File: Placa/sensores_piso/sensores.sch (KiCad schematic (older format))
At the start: 10 parts, among them P1 CONN_8X2, U1 CNY70, U2 CNY70

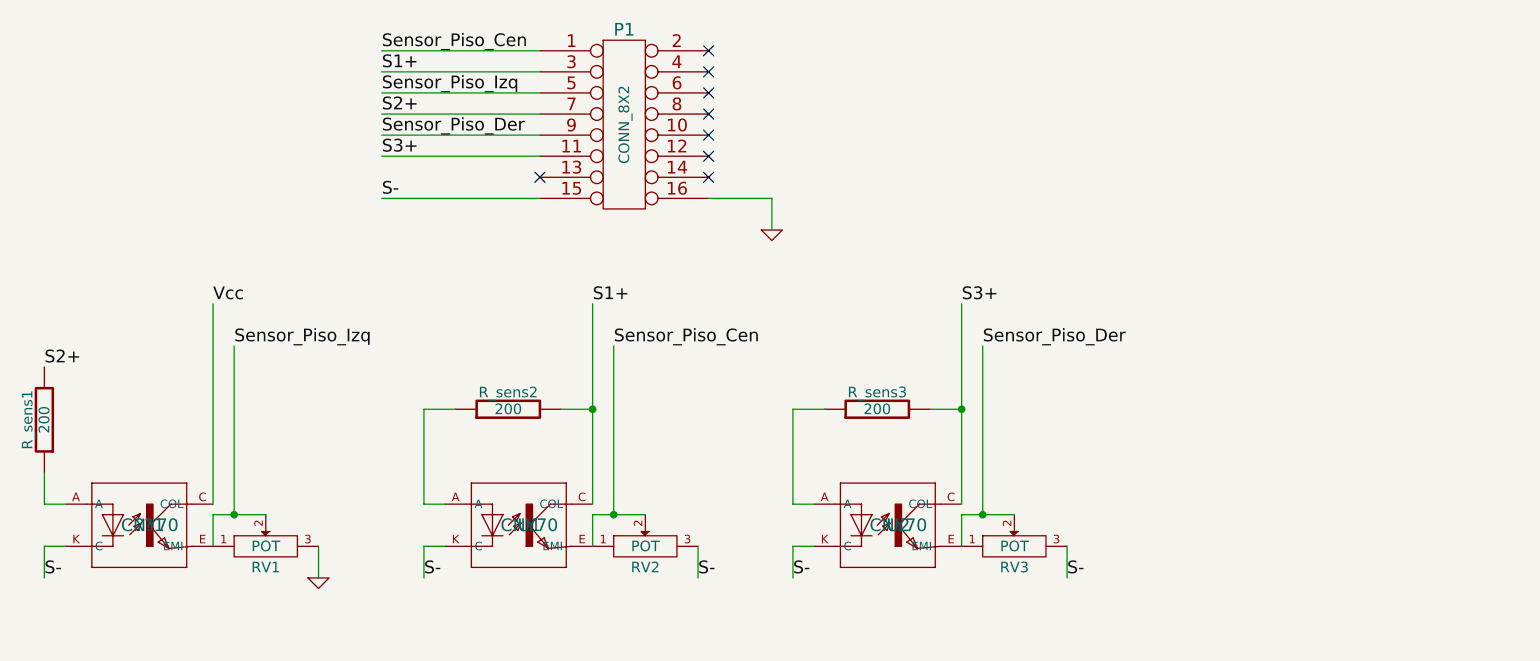
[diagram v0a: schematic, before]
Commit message: arreglo placa sensores
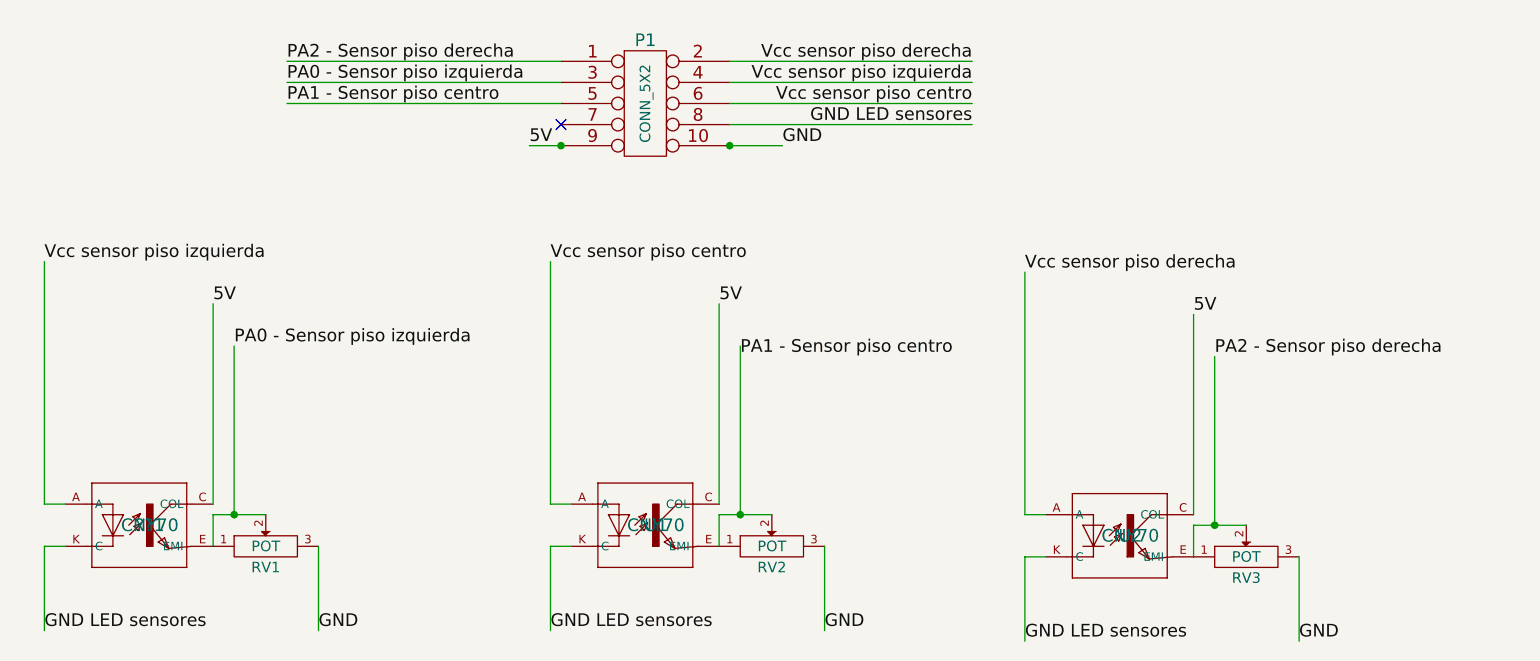
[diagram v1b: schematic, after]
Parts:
- removed P1: CONN_8X2, ~, symbol CONN_8X2
- removed R_sens1, R_sens2, R_sens3: 200, symbol R
- added P1: CONN_5X2, ~, symbol CONN_5X2
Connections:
- net S3+ is gone; now on net 5V: U2.C (COL)
- net Vcc is gone; now on net 5V: ??1.C (COL)
- net GND: now also RV2.3, RV3.3, P1.10
- net Vcc sensor piso izquierda: now reaches ??1.A
- net Vcc sensor piso izquierda: now also P1.4
- net Vcc sensor piso centro: now reaches U1.A
- net Vcc sensor piso centro: now also P1.6
- net Vcc sensor piso derecha: now reaches U2.A
- net Vcc sensor piso derecha: now also P1.2
- net S- renamed GND LED sensores
- net GND LED sensores: now also P1.8; no longer RV2.3, RV3.3
- net S1+ renamed 5V
- net 5V: now also P1.9
- net Sensor_Piso_Cen renamed PA1 - Sensor piso centro
- net PA1 - Sensor piso centro: now also P1.5
- net Sensor_Piso_Der renamed PA2 - Sensor piso derecha
- net PA2 - Sensor piso derecha: now also P1.1
- net Sensor_Piso_Izq renamed PA0 - Sensor piso izquierda
- net PA0 - Sensor piso izquierda: now also P1.3
- no-connect marks 8 -> 1
